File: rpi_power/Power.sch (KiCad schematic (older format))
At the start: 27 parts, among them U1 TPS54625

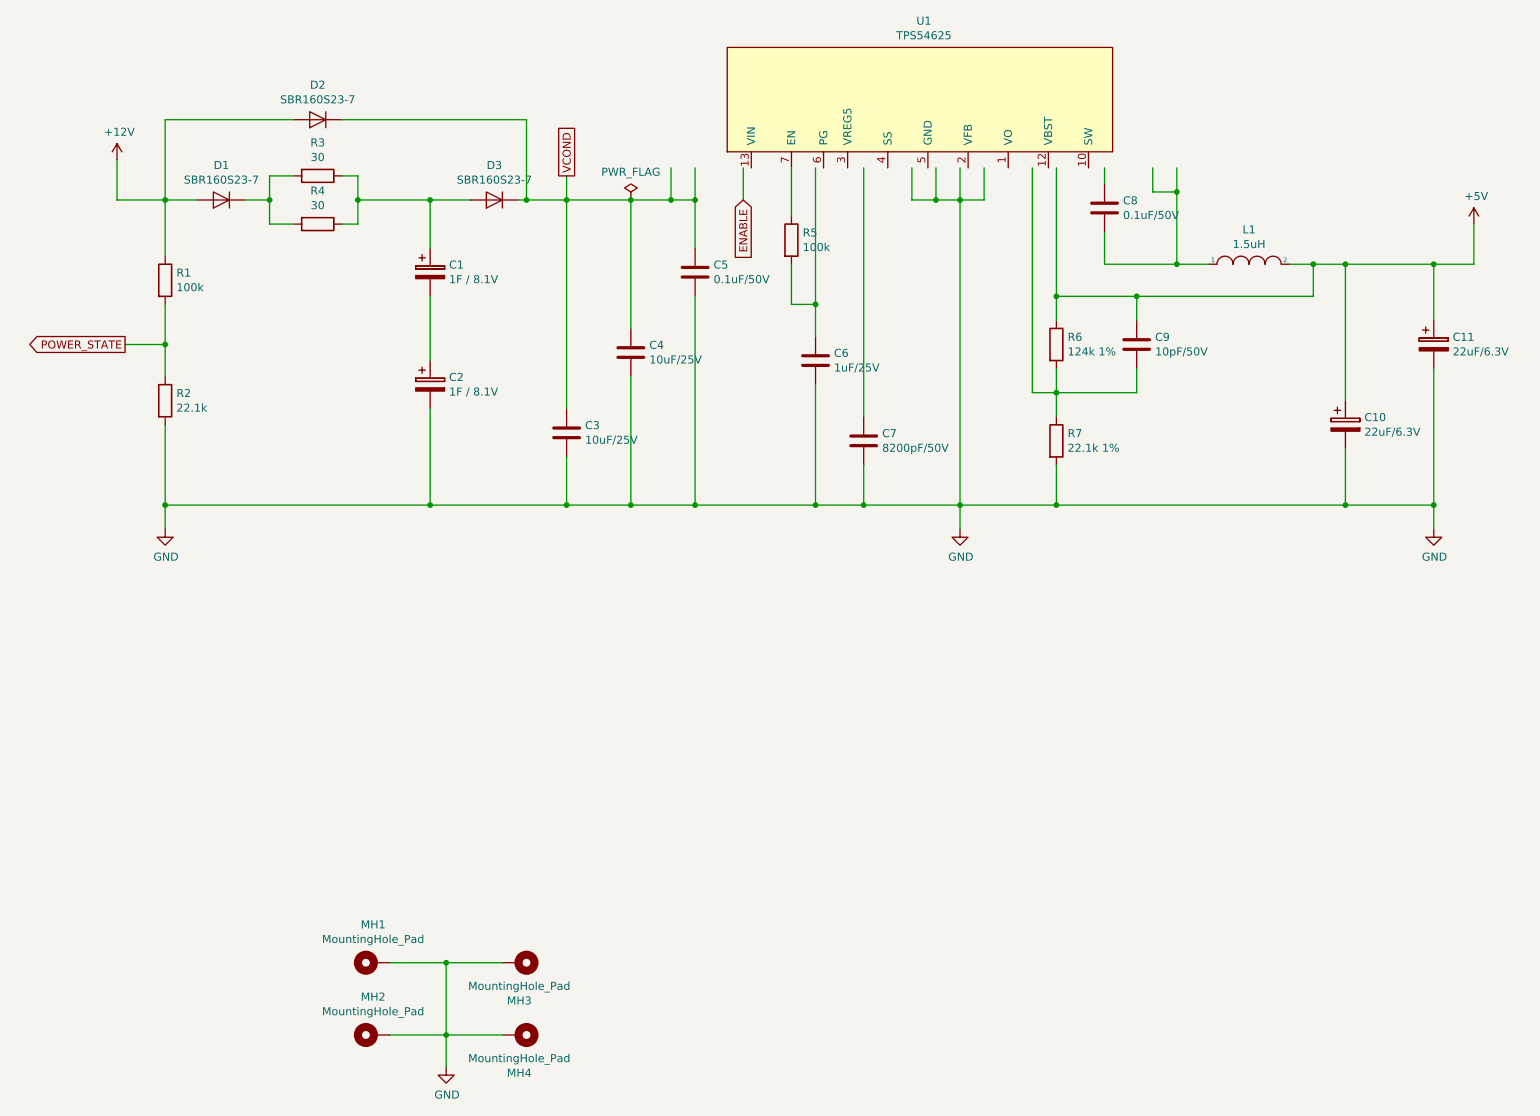
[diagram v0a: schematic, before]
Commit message: Routing done, pending review.
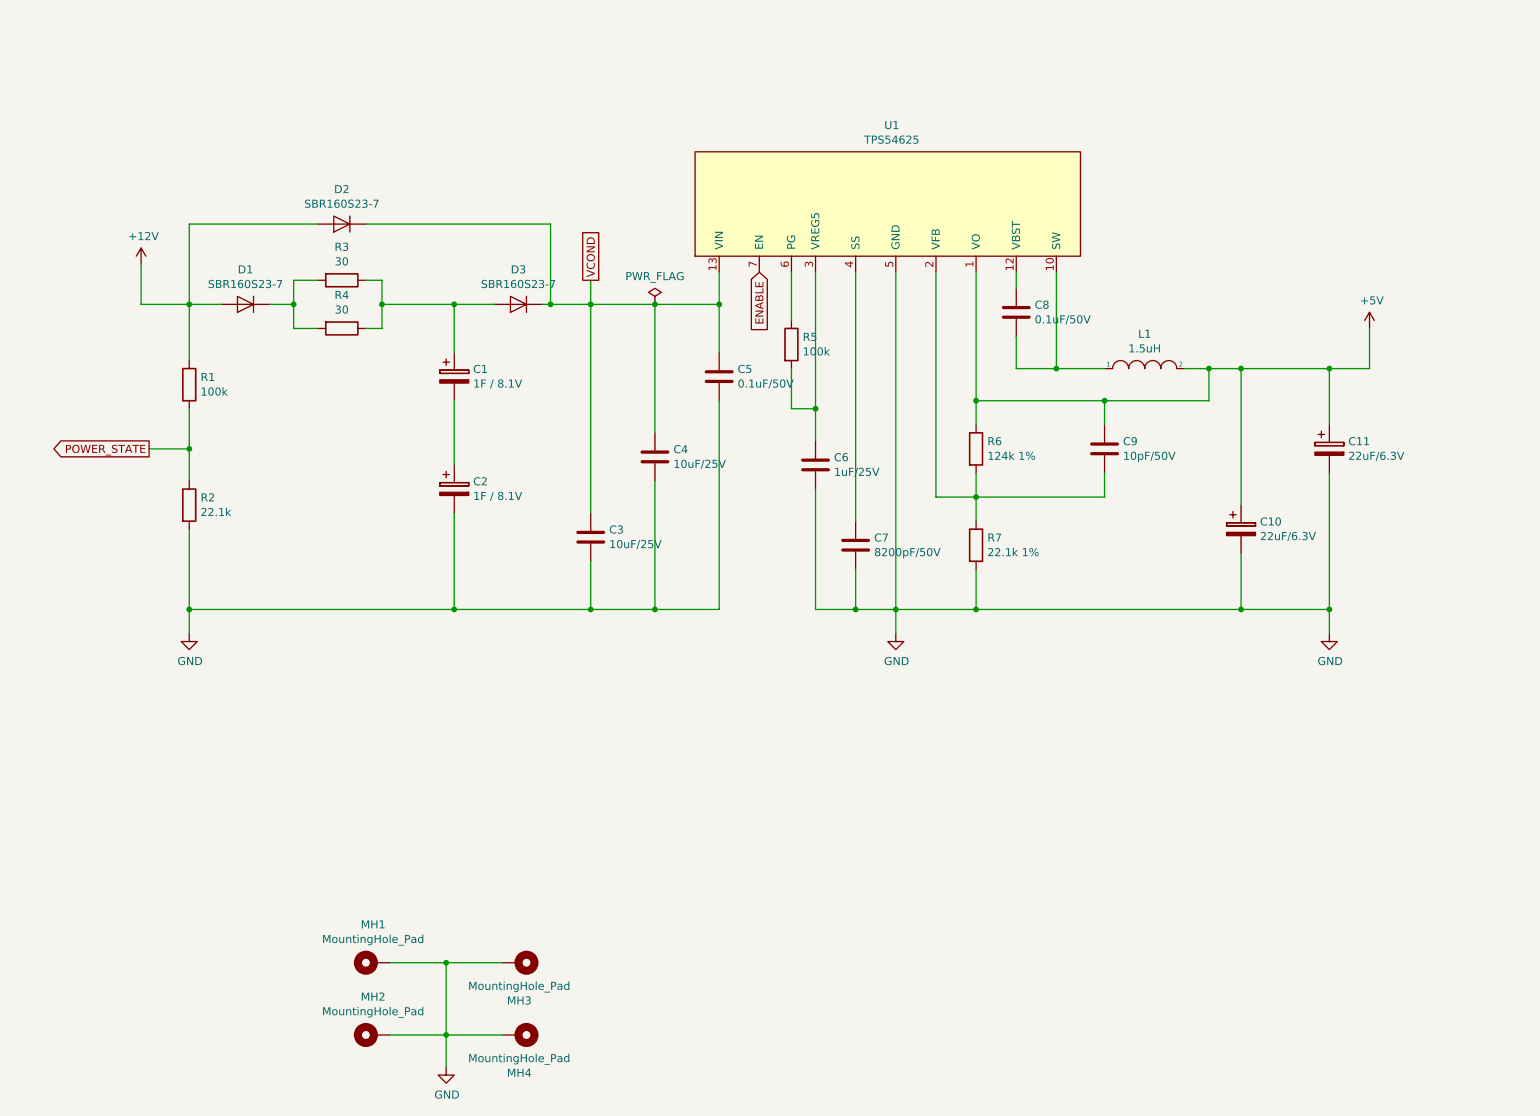
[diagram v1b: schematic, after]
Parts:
- U1: footprint TexasInstruments:HTSSOP-14-PWP -> TexasInstruments:HTSSOP-14-PWP_Handsolder
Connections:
- wire segments 106 -> 92
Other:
- moved on the sheet: C1, C10, C11, C2, C3, C4, C5, C6, C7, C8, C9, D1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
